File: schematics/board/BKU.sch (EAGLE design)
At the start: 73 parts, among them Q1 8MHz, Q2 32,768KHz, U1 STM32F405RGT6

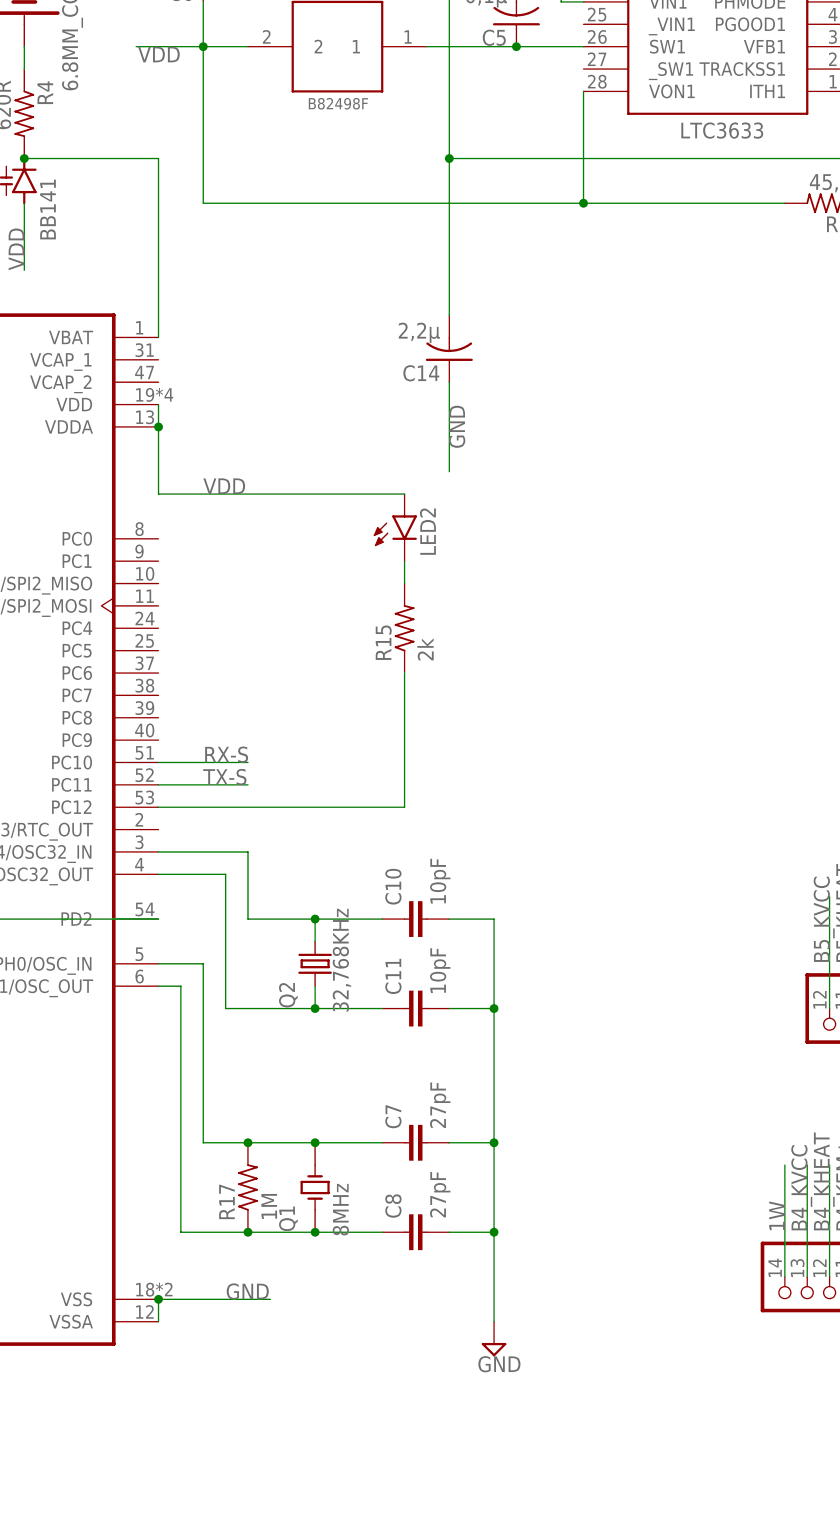
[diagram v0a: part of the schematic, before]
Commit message: Изменения в подключении мк
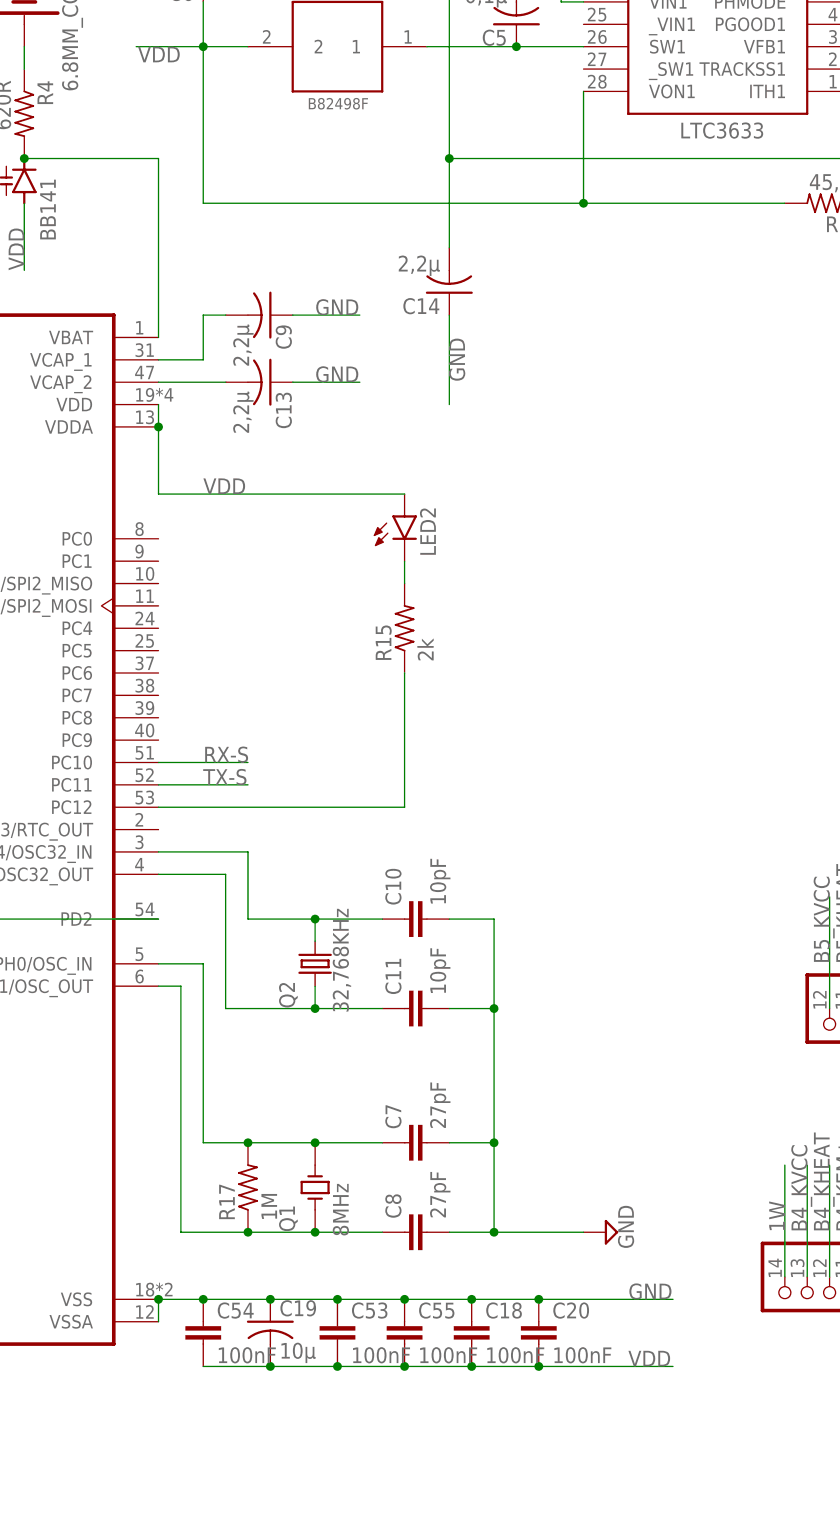
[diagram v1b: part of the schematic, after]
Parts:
- added C13, C9: 2,2µ, rcl:C-USC0603
- added C18, C20, C53, C54, C55: 100nF, rcl:C-EUC0603
- added C19: 10µ, rcl:C-USC1206
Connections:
- new net N$7: C9.2, U1.VCAP_1
- new net N$8: C13.2, U1.VCAP_2
- net GND: now also C13.1, C18.1, C19.1, C20.1, C53.1, C54.1, C55.1, C9.1
- net VDD: now also C18.2, C19.2, C20.2, C53.2, C54.2, C55.2
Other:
- moved on the sheet: C14
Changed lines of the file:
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@@
 <part name="JP1" library="pinheadCS" deviceset="PINHD-1X2" device=""/>
 <part name="R14" library="resistor" library_urn="urn:adsk.eagle:library:348" deviceset="R-US_" device="R0603" package3d_urn="urn:adsk.eagle:package:23555/3" value="10k"/>
+<part name="C9" library="rcl" library_urn="urn:adsk.eagle:library:334" deviceset="C-US" device="C0603" package3d_urn="urn:adsk.eagle:package:23616/2" value="2,2µ"/>
+<part name="C13" library="rcl" library_urn="urn:adsk.eagle:library:334" deviceset="C-US" device="C0603" package3d_urn="urn:adsk.eagle:package:23616/2" value="2,2µ"/>
+<part name="C18" library="rcl" library_urn="urn:adsk.eagle:library:334" deviceset="C-EU" device="C0603" package3d_urn="urn:adsk.eagle:package:23616/2" value="100nF"/>
+<part name="C53" library="rcl" library_urn="urn:adsk.eagle:library:334" deviceset="C-EU" device="C0603" package3d_urn="urn:adsk.eagle:package:23616/2" value="100nF"/>
+<part name="C54" library="rcl" library_urn="urn:adsk.eagle:library:334" deviceset="C-EU" device="C0603" package3d_urn="urn:adsk.eagle:package:23616/2" value="100nF"/>
+<part name="C19" library="rcl" library_urn="urn:adsk.eagle:library:334" deviceset="C-US" device="C1206" package3d_urn="urn:adsk.eagle:package:23618/2" value="10µ"/>
+<part name="C55" library="rcl" library_urn="urn:adsk.eagle:library:334" deviceset="C-EU" device="C0603" package3d_urn="urn:adsk.eagle:package:23616/2" value="100nF"/>
+<part name="C20" library="rcl" library_urn="urn:adsk.eagle:library:334" deviceset="C-EU" device="C0603" package3d_urn="urn:adsk.eagle:package:23616/2" value="100nF"/>
 </parts>
 <sheets>
@@
 <attribute name="VALUE" x="372.11" y="201.422" size="1.778" layer="96" rot="R180"/>
 </instance>
-<instance part="C14" gate="G$1" x="325.12" y="180.34" smashed="yes" rot="R180">
-<attribute name="NAME" x="324.104" y="179.705" size="1.778" layer="95" rot="R180"/>
-<attribute name="VALUE" x="324.104" y="184.531" size="1.778" layer="96" rot="R180"/>
+<instance part="C14" gate="G$1" x="325.12" y="187.96" smashed="yes" rot="R180">
+<attribute name="NAME" x="324.104" y="187.325" size="1.778" layer="95" rot="R180"/>
+<attribute name="VALUE" x="324.104" y="192.151" size="1.778" layer="96" rot="R180"/>
 </instance>
 <instance part="C6" gate="G$1" x="297.18" y="223.52" smashed="yes" rot="R180">
@@
 <attribute name="VALUE" x="324.739" y="82.804" size="1.778" layer="96" rot="R90"/>
 </instance>
-<instance part="SUPPLY22" gate="GND" x="330.2" y="68.58" smashed="yes">
-<attribute name="VALUE" x="328.295" y="65.405" size="1.778" layer="96"/>
+<instance part="SUPPLY22" gate="GND" x="342.9" y="81.28" smashed="yes" rot="R90">
+<attribute name="VALUE" x="346.075" y="79.375" size="1.778" layer="96" rot="R90"/>
 </instance>
 <instance part="Q2" gate="G$1" x="309.88" y="111.76" smashed="yes" rot="R90">
@@
 <attribute name="VALUE" x="207.01" y="109.982" size="1.778" layer="96" rot="R180"/>
 </instance>
+<instance part="C9" gate="G$1" x="304.8" y="185.42" smashed="yes" rot="R270">
+<attribute name="NAME" x="305.435" y="184.404" size="1.778" layer="95" rot="R270"/>
+<attribute name="VALUE" x="300.609" y="184.404" size="1.778" layer="96" rot="R270"/>
+</instance>
+<instance part="C13" gate="G$1" x="304.8" y="177.8" smashed="yes" rot="R270">
+<attribute name="NAME" x="305.435" y="176.784" size="1.778" layer="95" rot="R270"/>
+<attribute name="VALUE" x="300.609" y="176.784" size="1.778" layer="96" rot="R270"/>
+</instance>
+<instance part="C18" gate="G$1" x="327.66" y="71.12" smashed="yes">
+<attribute name="NAME" x="329.184" y="71.501" size="1.778" layer="95"/>
+<attribute name="VALUE" x="329.184" y="66.421" size="1.778" layer="96"/>
+</instance>
+<instance part="C53" gate="G$1" x="312.42" y="71.12" smashed="yes">
+<attribute name="NAME" x="313.944" y="71.501" size="1.778" layer="95"/>
+<attribute name="VALUE" x="313.944" y="66.421" size="1.778" layer="96"/>
+</instance>
+<instance part="C54" gate="G$1" x="297.18" y="71.12" smashed="yes">
+<attribute name="NAME" x="298.704" y="71.501" size="1.778" layer="95"/>
+<attribute name="VALUE" x="298.704" y="66.421" size="1.778" layer="96"/>
+</instance>
+<instance part="C19" gate="G$1" x="304.8" y="71.12" smashed="yes">
+<attribute name="NAME" x="305.816" y="71.755" size="1.778" layer="95"/>
+<attribute name="VALUE" x="305.816" y="66.929" size="1.778" layer="96"/>
+</instance>
+<instance part="C55" gate="G$1" x="320.04" y="71.12" smashed="yes">
+<attribute name="NAME" x="321.564" y="71.501" size="1.778" layer="95"/>
+<attribute name="VALUE" x="321.564" y="66.421" size="1.778" layer="96"/>
+</instance>
+<instance part="C20" gate="G$1" x="335.28" y="71.12" smashed="yes">
+<attribute name="NAME" x="336.804" y="71.501" size="1.778" layer="95"/>
+<attribute name="VALUE" x="336.804" y="66.421" size="1.778" layer="96"/>
+</instance>
 </instances>
 <busses>
@@
 </segment>
 <segment>
-<wire x1="325.12" y1="177.8" x2="325.12" y2="167.64" width="0.1524" layer="91"/>
-<label x="325.12" y="175.26" size="1.778" layer="95" rot="R270"/>
+<wire x1="325.12" y1="185.42" x2="325.12" y2="175.26" width="0.1524" layer="91"/>
+<label x="325.12" y="182.88" size="1.778" layer="95" rot="R270"/>
 <pinref part="C14" gate="G$1" pin="1"/>
 </segment>
@@
 <pinref part="C8" gate="G$1" pin="2"/>
 <wire x1="325.12" y1="81.28" x2="330.2" y2="81.28" width="0.1524" layer="91"/>
-<wire x1="330.2" y1="81.28" x2="330.2" y2="71.12" width="0.1524" layer="91"/>
+<wire x1="330.2" y1="81.28" x2="340.36" y2="81.28" width="0.1524" layer="91"/>
 <pinref part="C11" gate="G$1" pin="2"/>
 <wire x1="325.12" y1="106.68" x2="330.2" y2="106.68" width="0.1524" layer="91"/>
@@
 <segment>
 <pinref part="U1" gate="G$1" pin="VSS"/>
-<wire x1="292.1" y1="73.66" x2="304.8" y2="73.66" width="0.1524" layer="91"/>
-<label x="299.72" y="73.66" size="1.778" layer="95"/>
+<label x="345.44" y="73.66" size="1.778" layer="95"/>
 <pinref part="U1" gate="G$1" pin="VSSA"/>
+<wire x1="292.1" y1="73.66" x2="297.18" y2="73.66" width="0.1524" layer="91"/>
+<wire x1="297.18" y1="73.66" x2="304.8" y2="73.66" width="0.1524" layer="91"/>
+<wire x1="304.8" y1="73.66" x2="312.42" y2="73.66" width="0.1524" layer="91"/>
+<wire x1="312.42" y1="73.66" x2="320.04" y2="73.66" width="0.1524" layer="91"/>
+<wire x1="320.04" y1="73.66" x2="327.66" y2="73.66" width="0.1524" layer="91"/>
+<wire x1="327.66" y1="73.66" x2="335.28" y2="73.66" width="0.1524" layer="91"/>
+<wire x1="335.28" y1="73.66" x2="350.52" y2="73.66" width="0.1524" layer="91"/>
 <wire x1="292.1" y1="71.12" x2="292.1" y2="73.66" width="0.1524" layer="91"/>
 <junction x="292.1" y="73.66"/>
+<pinref part="C18" gate="G$1" pin="1"/>
+<junction x="327.66" y="73.66"/>
+<pinref part="C53" gate="G$1" pin="1"/>
+<junction x="312.42" y="73.66"/>
+<pinref part="C54" gate="G$1" pin="1"/>
+<junction x="297.18" y="73.66"/>
+<pinref part="C55" gate="G$1" pin="1"/>
+<junction x="320.04" y="73.66"/>
+<pinref part="C19" gate="G$1" pin="1"/>
+<junction x="304.8" y="73.66"/>
+<pinref part="C20" gate="G$1" pin="1"/>
+<junction x="335.28" y="73.66"/>
 </segment>
 <segment>
@@
 <label x="195.58" y="106.68" size="1.778" layer="95" rot="R180"/>
 </segment>
+<segment>
+<wire x1="307.34" y1="185.42" x2="314.96" y2="185.42" width="0.1524" layer="91"/>
+<label x="309.88" y="185.42" size="1.778" layer="95"/>
+<pinref part="C9" gate="G$1" pin="1"/>
+</segment>
+<segment>
+<wire x1="307.34" y1="177.8" x2="314.96" y2="177.8" width="0.1524" layer="91"/>
+<label x="309.88" y="177.8" size="1.778" layer="95"/>
+<pinref part="C13" gate="G$1" pin="1"/>
+</segment>
 </net>
 <net name="5V" class="0">
@@
 <label x="195.58" y="116.84" size="1.778" layer="95" rot="R180"/>
 </segment>
+<segment>
+<wire x1="350.52" y1="66.04" x2="335.28" y2="66.04" width="0.1524" layer="91"/>
+<pinref part="C18" gate="G$1" pin="2"/>
+<junction x="327.66" y="66.04"/>
+<wire x1="335.28" y1="66.04" x2="327.66" y2="66.04" width="0.1524" layer="91"/>
+<wire x1="327.66" y1="66.04" x2="320.04" y2="66.04" width="0.1524" layer="91"/>
+<pinref part="C53" gate="G$1" pin="2"/>
+<wire x1="320.04" y1="66.04" x2="312.42" y2="66.04" width="0.1524" layer="91"/>
+<wire x1="312.42" y1="66.04" x2="304.8" y2="66.04" width="0.1524" layer="91"/>
+<junction x="312.42" y="66.04"/>
+<pinref part="C55" gate="G$1" pin="2"/>
+<junction x="320.04" y="66.04"/>
+<pinref part="C19" gate="G$1" pin="2"/>
+<pinref part="C54" gate="G$1" pin="2"/>
+<wire x1="304.8" y1="66.04" x2="297.18" y2="66.04" width="0.1524" layer="91"/>
+<junction x="304.8" y="66.04"/>
+<label x="345.44" y="66.04" size="1.778" layer="95"/>
+<pinref part="C20" gate="G$1" pin="2"/>
+<junction x="335.28" y="66.04"/>
+</segment>
 </net>
 <net name="N$24" class="0">
@@
 <wire x1="340.36" y1="226.06" x2="325.12" y2="226.06" width="0.1524" layer="91"/>
 <junction x="325.12" y="226.06"/>
-<wire x1="325.12" y1="203.2" x2="325.12" y2="185.42" width="0.1524" layer="91"/>
+<wire x1="325.12" y1="203.2" x2="325.12" y2="193.04" width="0.1524" layer="91"/>
 <junction x="325.12" y="203.2"/>
 <pinref part="C14" gate="G$1" pin="2"/>
@@
 </segment>
 </net>
+<net name="N$8" class="0">
+<segment>
+<pinref part="C13" gate="G$1" pin="2"/>
+<wire x1="292.1" y1="177.8" x2="299.72" y2="177.8" width="0.1524" layer="91"/>
+<pinref part="U1" gate="G$1" pin="VCAP_2"/>
+</segment>
+</net>
+<net name="N$7" class="0">
+<segment>
+<pinref part="C9" gate="G$1" pin="2"/>
+<wire x1="299.72" y1="185.42" x2="297.18" y2="185.42" width="0.1524" layer="91"/>
+<wire x1="297.18" y1="185.42" x2="297.18" y2="180.34" width="0.1524" layer="91"/>
+<pinref part="U1" gate="G$1" pin="VCAP_1"/>
+<wire x1="297.18" y1="180.34" x2="292.1" y2="180.34" width="0.1524" layer="91"/>
+</segment>
+</net>
